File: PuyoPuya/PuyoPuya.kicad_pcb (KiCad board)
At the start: 2 copper layers, 8.7 x 4.5 mm, 17 parts, among them J1 Conn_01x10, J2 SWD, J3 USB4085-GF-A, SW1 SW_Push, U1 PY32F003W16S6TU

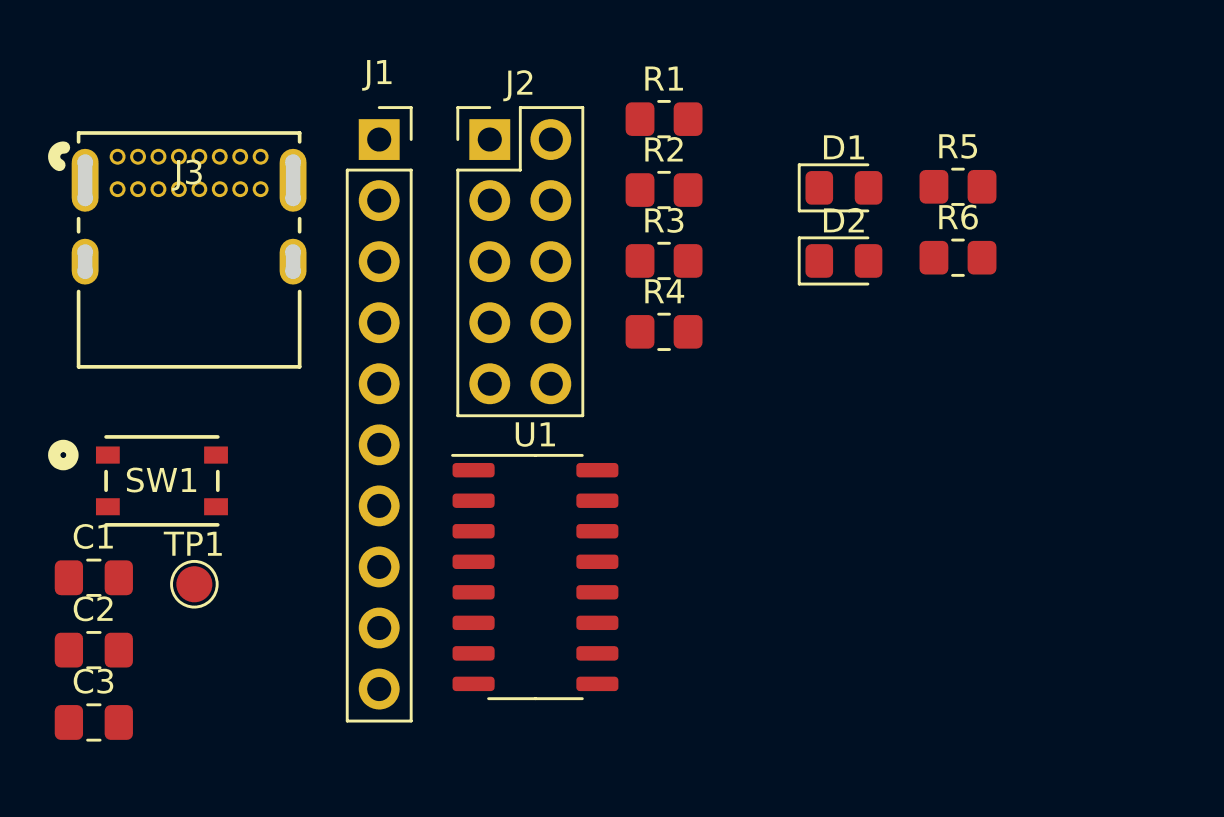
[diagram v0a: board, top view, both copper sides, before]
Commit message: Boarb
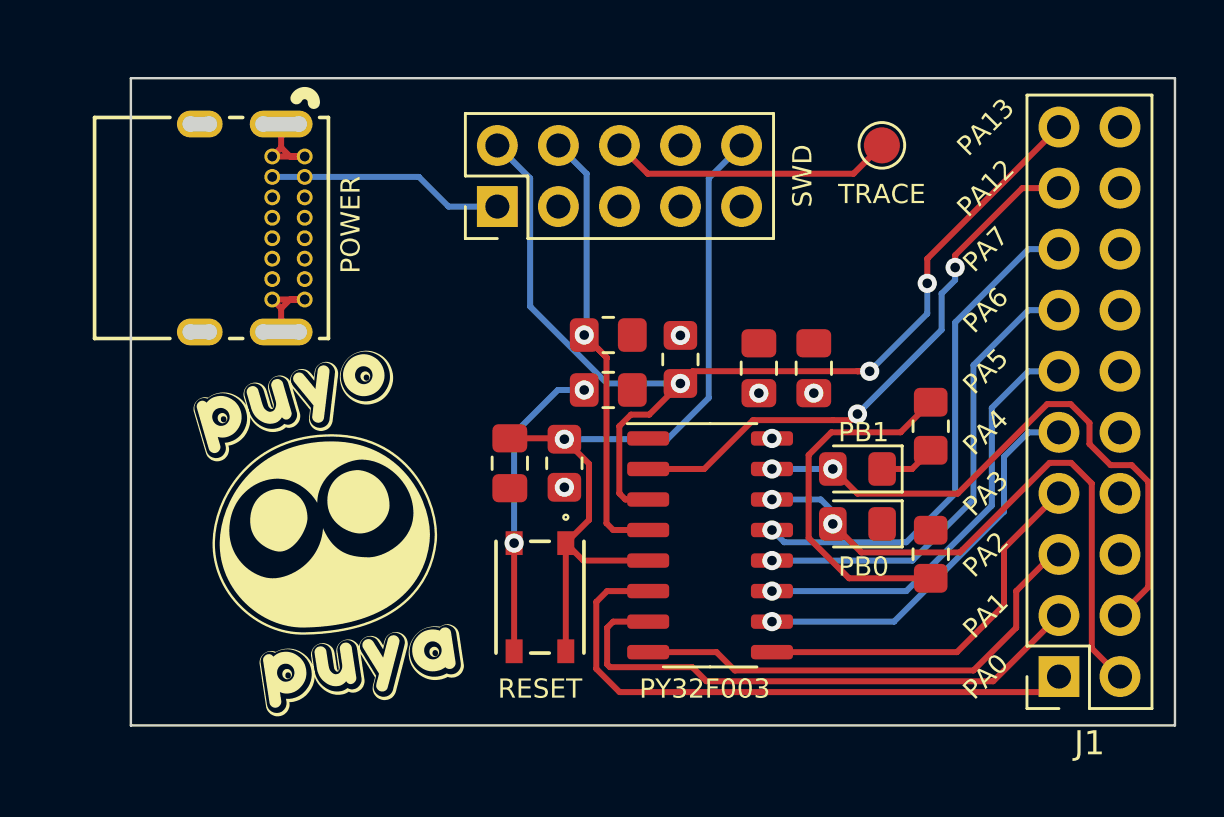
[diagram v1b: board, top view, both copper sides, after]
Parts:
- J1: value Conn_01x10 -> Conn_02x10; footprint Connector_PinSocket_2.54mm:PinSocket_1x10_P2.54mm_Vertical -> Connector_PinSocket_2.54mm:PinSocket_2x10_P2.54mm_Vertical
- moved J1 36.0 mm to (156.7, 74.9), turned to 180 degrees
- moved TP1 33.9 mm to (149.4, 52.8)
- moved C2 32.2 mm to (146.5, 62.1), turned to 90 degrees
- moved C1 29.0 mm to (144.2, 62.1), turned to 90 degrees
- moved C3 20.4 mm to (133.9, 66.1), turned to -90 degrees
- moved SW1 16.5 mm to (135.1, 71.6), turned to -90 degrees
- moved R5 15.3 mm to (151.4, 69.8), turned to 90 degrees
- moved D1 14.0 mm to (148.3, 68.6), turned to 180 degrees
- moved R1 10.0 mm to (141.0, 61.7), turned to -90 degrees
- moved R3 9.38 mm to (136.1, 66.1), turned to 90 degrees
- moved D2 8.67 mm to (148.3, 66.3), turned to 180 degrees
- moved J3 7.78 mm to (125.3, 53.3), turned to -90 degrees
- moved U1 7.38 mm to (142.2, 69.5)
- moved R6 7.10 mm to (151.4, 64.5), turned to -90 degrees
- moved R2 6.46 mm to (138.0, 60.7)
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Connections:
- J1 pad 10: /PA13/SWDIO -> VCC
- J1 pad 2: /PA1 -> /PB0
- J1 pad 3: /PA2 -> /PA1
- J1 pad 4: /PA3 -> /PB1
- J1 pad 5: /PA4 -> /PA2
- J1 pad 6: /PA5 -> VCC
- J1 pad 7: /PA6 -> /PA3
- J1 pad 8: /PA7 -> VCC
- J1 pad 9: /PA12 -> /PA4
- J2 pad 4: /SWCLK -> /SWDCLK
- J3 pad B12: unconnected-(J3-GND-PadB12) -> GND
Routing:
- net /PA13/SWDIO: track 0.00 -> 44.2 mm, vias 0 -> 3
- net /NRST: track 0.00 -> 33.4 mm, vias 0 -> 1
- net /PB1: track 0.00 -> 25.5 mm, vias 0 -> 2
- net /PA0: track 0.00 -> 25.0 mm
- net /PB0: track 0.00 -> 24.9 mm, vias 0 -> 2
- net /PA1: track 0.00 -> 23.6 mm
- net /PA12: track 0.00 -> 23.4 mm, vias 0 -> 2
- net GND: track 0.00 -> 23.0 mm
- net /PA7: track 0.00 -> 21.4 mm, vias 0 -> 1
- net /PA2: track 0.00 -> 20.3 mm
- net /PA6: track 0.00 -> 19.5 mm, vias 0 -> 1
- net /SWDCLK: track 0.00 -> 19.0 mm, vias 0 -> 1
- net /PA5: track 0.00 -> 18.1 mm, vias 0 -> 1
- net /PA4: track 0.00 -> 16.5 mm, vias 0 -> 1
- net /PA3: track 0.00 -> 16.1 mm
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- added copper zone on F.Cu, net GND
- added copper zone on B.Cu, net VCC
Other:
- board size 8.7 x 4.5 mm -> 43.4 x 26.9 mm
- board text added: "PA0"
- board text added: "PA1"
- board text added: "PA12"
- board text added: "PA13"
- board text added: "PA2"
- board text added: "PA3"
- board text added: "PA4"
- board text added: "PA5"
- board text added: "PA6"
- board text added: "PA7"
- board text added: "PB0"
- board text added: "PB1"
- board text added: "POWER"
- board text added: "PY32F003"
- board text added: "RESET"
- board text added: "SWD"
- board text added: "TRACE"
